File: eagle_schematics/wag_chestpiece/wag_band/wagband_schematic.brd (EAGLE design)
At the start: 100 x 80 mm, 8 parts, among them U2 TLV1117-33CDCY

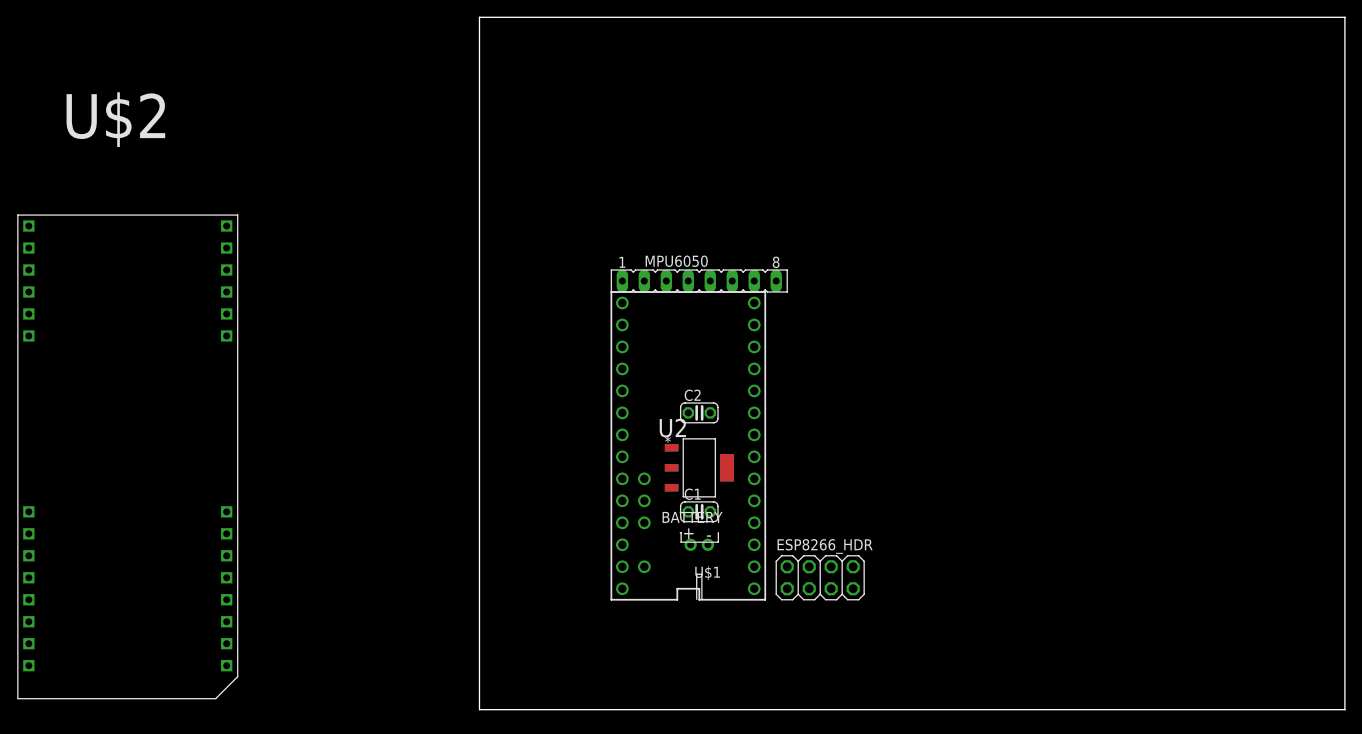
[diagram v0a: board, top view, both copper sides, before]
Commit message: Added more parts for eagle
Finished PCBs
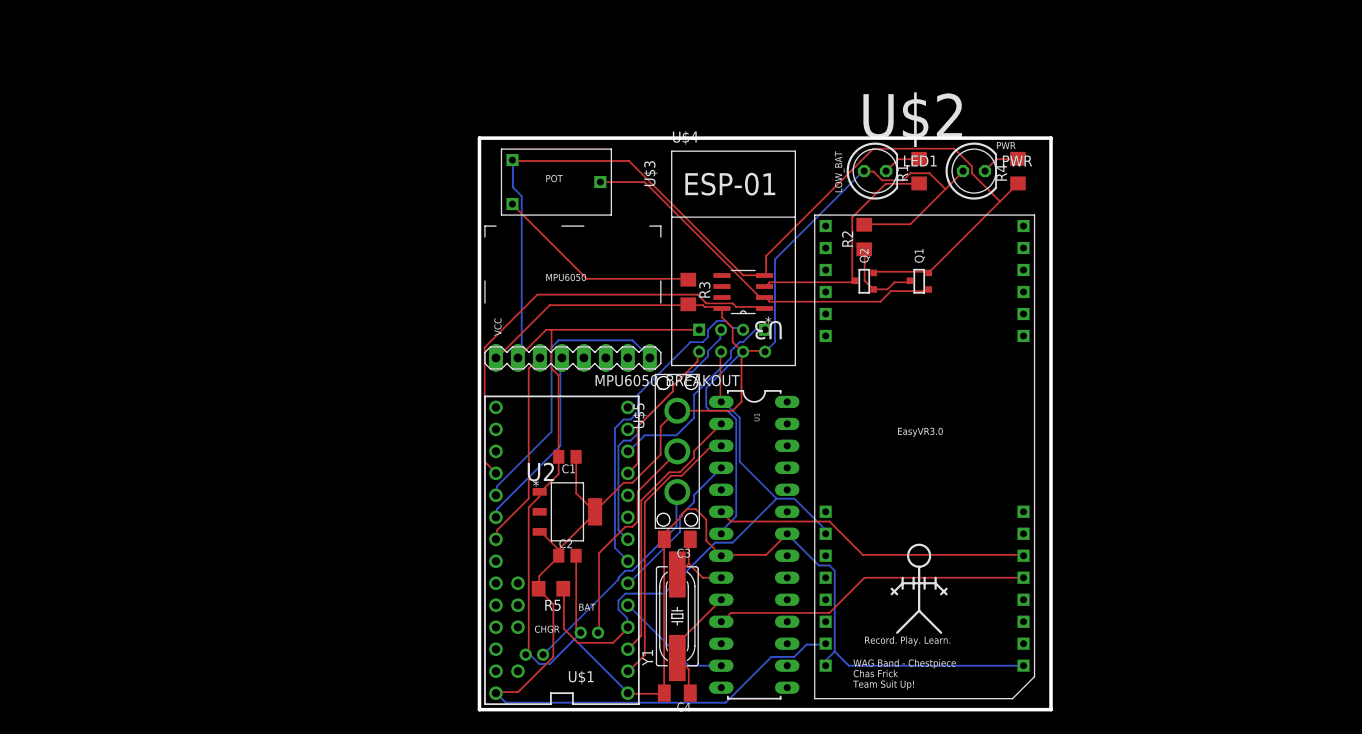
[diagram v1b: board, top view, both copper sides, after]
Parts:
- removed BATTERY: (no value), adafruit:JST-PH-2-THM-RA
- removed ESP8266_HDR: (no value), pinhead:2X04
- removed MPU6050: (no value), con-lsta:FE08
- added BAT, CHGR: (no value), adafruit:JST-PH-2-THM-RA
- added C3, C4: 22pF, rcl:C1206K
- added LED1, PWR: (no value), led:LED5MM
- added MPU6050_BREAKOUT: (no value), mqp_custom_parts:MPU6050
- added Q1, Q2: (no value), mqp_custom_parts:SOT-23
- added R1, R4: 1k, resistor:R1206
- added R2, R3: 30k, resistor:R1206
- added R5: 10k, resistor:R1206
- added U$3: CB10LV103M, mqp_custom_parts:CB10
- added U$4: ESP01, esp8266modules:ESP01
- added U$5: MS12ASW13, mqp_custom_parts:SPDT
- added U1: ATMEGA328P_PDIP, SparkFun-DigitalIC:DIL28-3
- added U3: LM358DR, Texas Instruments_By_element14_Batch_1:SOIC127P600X175-8N
- added Y1: 16MHz, SparkFun-FreqCtrl:HC49UP
- C1, C2: device rcl:C025-024X044 -> resistor:C0805K
- moved U$2 92.1 mm to (51.4, 30.5)
- moved C2 22.5 mm to (10.2, 17.8)
- moved U$1 18.9 mm to (9.53, 18.4)
- moved C1 16.5 mm to (10.2, 29.2), turned to 180 degrees
- moved U2 16.1 mm to (10.2, 22.9)
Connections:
- new net !RST: R5.1, U$1.2, U$2.P$8, U$4.CH_PD, U1.1
- new net N$10: Q2.3, R1.1, U3.3
- new net N$11: R3.1, U$3.P$2
- new net N$12: LED1.K, R1.2
- new net N$13: U$1.1, U1.2
- new net N$14: U$1.16/A2, U3.1
- new net N$15: PWR.K, R4.2
- new net N$16: U$1.3, U1.13
- new net N$18: U$1.6, U$4.GPIO2
- new net N$20: C3.1, U1.9, Y1.2
- new net N$22: U$1.0, U1.3
- new net N$23: BAT.1, U$5.P$2
- new net N$25: CHGR.1, U$5.P$3
- new net N$3: MPU6050_BREAKOUT.SDA, U$1.18/A4
- new net N$6: U$2.P$20, U1.6
- new net N$9: Q1.3, Q2.1, R2.1
- net GND: now also BAT.2, C3.2, C4.2, CHGR.2, MPU6050_BREAKOUT.GND, Q1.2, Q2.2, R4.1, U$3.P$1, U$4.GND, U1.22, U1.8, U3.4; no longer BATTERY.1, ESP8266_HDR.2, MPU6050.2
- net N$1: now also U$1.4, U1.4; no longer U$1.7, U$2.P$20
- net N$17: now also MPU6050_BREAKOUT.SCL; no longer MPU6050.3
- net N$19: now also U$1.9, U$4.TX; no longer ESP8266_HDR.8, U$1.1
- net N$2: now also U$1.10, U$4.RX; no longer U$1.8, U$2.P$19
- net N$21: now also C4.1, U1.10, Y1.1; no longer ESP8266_HDR.5, U$1.2
- net N$4: now also Q1.1, U$3.P$3, U3.2; no longer MPU6050.4, U$1.18/A4
- net N$5: now also U$2.P$19, U1.11; no longer U$1.3, U$2.P$8
- net N$7: now also U$1.5, U$4.GPIO0; no longer ESP8266_HDR.1, U$1.0
- net N$8: now also MPU6050_BREAKOUT.INT; no longer MPU6050.8
- net VCC: now also LED1.A, MPU6050_BREAKOUT.VCC, PWR.A, R2.2, R3.2, R5.2, U$4.RST, U$4.VCC, U$5.P$1, U1.7, U3.8; no longer BATTERY.2, ESP8266_HDR.3, ESP8266_HDR.7, MPU6050.1
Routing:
- net GND: track 0.00 -> 289.0 mm
- net VCC: track 0.00 -> 225.4 mm
- net !RST: track 0.00 -> 67.9 mm
- net N$14: track 0.00 -> 50.7 mm
- net N$4: track 0.00 -> 44.3 mm
- net N$7: track 0.00 -> 38.0 mm
- net N$6: track 0.00 -> 37.0 mm
- net N$5: track 0.00 -> 37.0 mm
- net N$8: track 0.00 -> 32.4 mm
- net N$22: track 0.00 -> 31.9 mm
- net N$13: track 0.00 -> 31.2 mm
- net N$18: track 0.00 -> 30.5 mm
- net N$10: track 0.00 -> 28.0 mm
- net N$25: track 0.00 -> 25.7 mm
- net N$23: track 0.00 -> 25.2 mm
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- added copper zone on layer 1, net GND
- added copper zone on layer 16, net GND
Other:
- board size 100 x 80 mm -> 66 x 66 mm
- board text added: "BAT"
- board text added: "CHGR"
- board text added: "EasyVR3.0"
- board text added: "LOW_BAT"
- board text added: "MPU6050"
- board text added: "POT"
- board text added: "PWR"
- board text added: "Record. Play. Learn."
- board text added: "VCC"
- board text added: "WAG Band - Chestpiece Chas Frick Team Suit Up!"
